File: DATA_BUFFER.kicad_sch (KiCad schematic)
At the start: 9 parts, among them IC301 ${DEVICE}

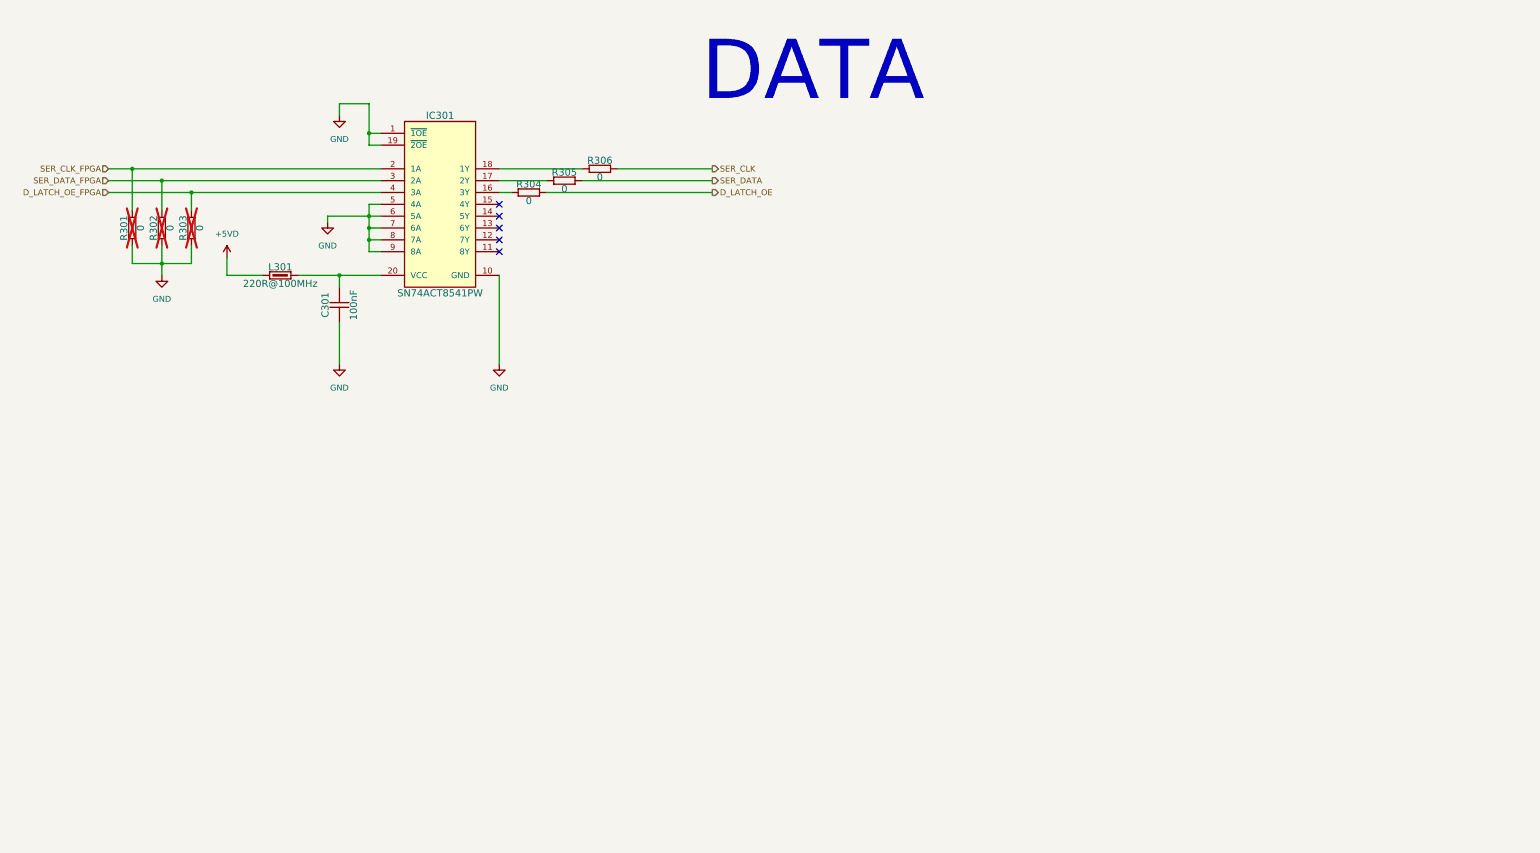
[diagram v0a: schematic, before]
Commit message: WIP snapshot
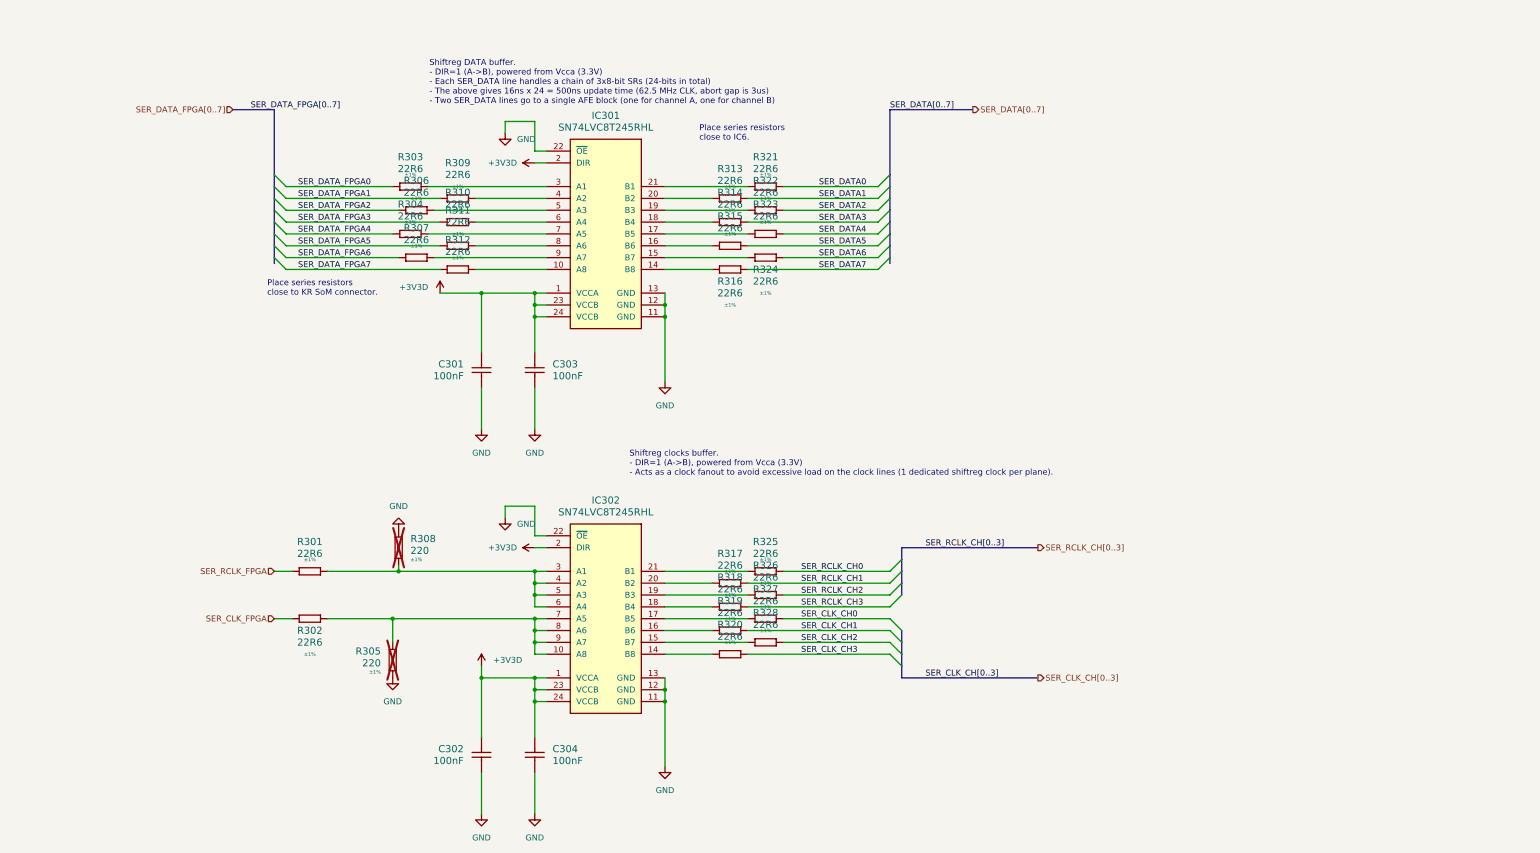
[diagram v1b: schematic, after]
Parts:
- removed IC301: ${DEVICE}, ICs And Semiconductors SMD:SOP65P640X120-20N, symbol CERN:Standard Logic/SN74ACT8541PW
- removed L301: 220R@100MHz, Inductors SMD:INDC1608X95N, symbol CERN:Inductors SMD/IND0603_MURATA_BLM18SG221TN1 [alt]
- removed R301, R302, R303, R304, R305, R306: 0, Resistors SMD:RESC1005X40N, symbol CERN:Resistors SMD/R0402_0R_JUMPER
- added C301, C302, C304: 100nF, Capacitors SMD:CAPC1005X55N, symbol CERN:Capacitors SMD/CC0402_100NF_25V_10%_X7R_YUDEN_TMK105B7104KVHF
- added IC301, IC302: ${DEVICE}, ICs And Semiconductors SMD:TEXAS_RHL (S-PVQFN-N24), symbol CERN_Linux:Standard Logic/SN74LVC8T245RHL
- added R301, R302, R303, R304, R306, R307, R309, R310, R311, R312, R313, R314, R315, R316, R317, R318, R319, R320, R321, R322, R323, R324, R325, R326, R327, R328: 22R6, Resistors SMD:RESC1005X40N, symbol CERN:Resistors SMD/R0402_22R6_1%_0.063W_100PPM
- added R305, R308: 220, Resistors SMD:RESC1005X40N, symbol CERN:Resistors SMD/R0402_220R_1%_0.0625W_100PPM
- renumbered C301 to C303
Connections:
- net GND: now also C301.1, C302.1, C304.1, IC301.11 (GND), IC301.12 (GND), IC301.13 (GND), IC301.22 (~{OE}), IC302.11 (GND), IC302.12 (GND), IC302.13 (GND), IC302.22 (~{OE}), R305.1, R308.1
- net SER_CLK_FPGA: now also R302.1
- net +3V3D: now reaches C303.2
- net +3V3D: now also C301.2, C302.2, C304.2, IC301.1 (VCCA), IC301.2 (DIR), IC301.23 (VCCB), IC301.24 (VCCB), IC302.1 (VCCA), IC302.2 (DIR), IC302.23 (VCCB), IC302.24 (VCCB)
- new net: IC302.10 (A8), IC302.7 (A5), IC302.8 (A6), IC302.9 (A7), R302.2, R305.2
- new net: IC301.9 (A7), R307.2
- new net: IC301.8 (A6), R311.2
- new net: IC301.3 (A1), R303.2
- new net: IC301.20 (B2), R313.1
- new net: IC301.21 (B1), R321.1
- new net: IC302.21 (B1), R325.1
- new net: IC301.14 (B8), R316.1
- new net: IC302.3 (A1), IC302.4 (A2), IC302.5 (A3), IC302.6 (A4), R301.2, R308.2
- new net: IC301.17 (B5), R323.1
- new net: IC302.16 (B6), R319.1
- new net: IC301.5 (A3), R306.2
- new net: IC301.18 (B4), R314.1
- new net: IC302.14 (B8), R320.1
- new net: IC302.15 (B7), R328.1
- new net: IC302.17 (B5), R327.1
- new net: IC302.18 (B4), R318.1
- new net: IC302.19 (B3), R326.1
- new net: IC302.20 (B2), R317.1
- new net: IC301.10 (A8), R312.2
- new net: IC301.6 (A4), R310.2
- new net: IC301.19 (B3), R322.1
- new net: IC301.4 (A2), R309.2
- new net: IC301.15 (B7), R324.1
- new net: IC301.16 (B6), R315.1
- new net: IC301.7 (A5), R304.2
- new net SER_CLK_CH0: R327.2
- new net SER_CLK_CH1: R319.2
- new net SER_CLK_CH2: R328.2
- new net SER_CLK_CH3: R320.2
- new net SER_DATA0: R321.2
- new net SER_DATA1: R313.2
- new net SER_DATA2: R322.2
- new net SER_DATA3: R314.2
- new net SER_DATA4: R323.2
- new net SER_DATA5: R315.2
- new net SER_DATA6: R324.2
- new net SER_DATA7: R316.2
- new net SER_DATA_FPGA0: R303.1
- new net SER_DATA_FPGA1: R309.1
- new net SER_DATA_FPGA2: R306.1
- new net SER_DATA_FPGA3: R310.1
- new net SER_DATA_FPGA4: R304.1
- new net SER_DATA_FPGA5: R311.1
- new net SER_DATA_FPGA6: R307.1
- new net SER_DATA_FPGA7: R312.1
- new net SER_RCLK_CH0: R325.2
- new net SER_RCLK_CH1: R317.2
- new net SER_RCLK_CH2: R326.2
- new net SER_RCLK_CH3: R318.2
- new net SER_RCLK_FPGA: R301.1
- no-connect marks 5 -> 0
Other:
- note added: "Place series resistors close to IC6."
- note added: "Place series resistors close to KR SoM connector."
- note added: "Shiftreg DATA buffer. - DIR=1 (A->B), powered from Vcca (3.3V) - Each SER_DATA line handles a chain of 3x8-bit SRs (24-bits in total) - The above gives 16ns x 24 = 500ns update time (62.5 MHz CLK, abort gap is 3us) - Two SER_DATA lines go to a single AFE block (one for channel A, one for channel B)"
- note added: "Shiftreg clocks buffer. - DIR=1 (A->B), powered from Vcca (3.3V) - Acts as a clock fanout to avoid excessive load on the clock lines (1 dedicated shiftreg clock per plane)."
- note removed: "DATA"
- moved on the sheet: C303

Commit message: Update project files and backups
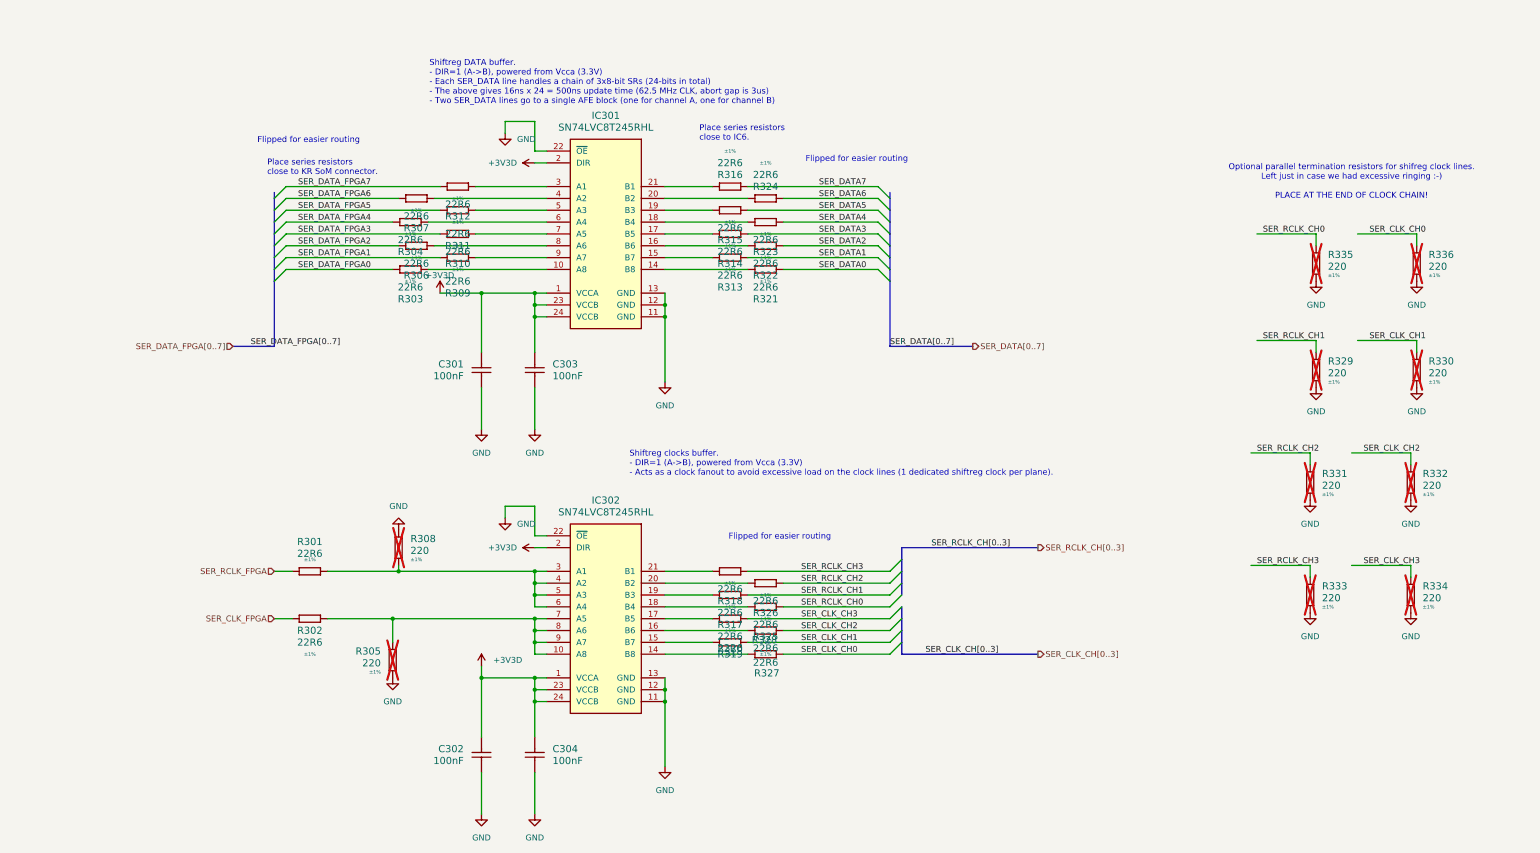
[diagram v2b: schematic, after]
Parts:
- added R329, R330, R331, R332, R333, R334, R335, R336: 220, Resistors SMD:RESC1005X40N, symbol CERN:Resistors SMD/R0402_220R_1%_0.0625W_100PPM
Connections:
- net GND: now also R329.1, R330.1, R331.1, R332.1, R333.1, R334.1, R335.1, R336.1
- net SER_CLK_CH0: now also R336.2
- net SER_CLK_CH1: now also R330.2
- net SER_CLK_CH2: now also R332.2
- net SER_CLK_CH3: now also R334.2
- net SER_RCLK_CH0: now also R335.2
- net SER_RCLK_CH1: now also R329.2
- net SER_RCLK_CH2: now also R331.2
- net SER_RCLK_CH3: now also R333.2
- net at R307.2: now also IC301.4 (A2); no longer IC301.9 (A7)
- net at R311.2: now also IC301.5 (A3); no longer IC301.8 (A6)
- net at R303.2: now also IC301.10 (A8); no longer IC301.3 (A1)
- net at R313.1: now also IC301.15 (B7); no longer IC301.20 (B2)
- net at R321.1: now also IC301.14 (B8); no longer IC301.21 (B1)
- net at R325.1: now also IC302.18 (B4); no longer IC302.21 (B1)
- net at R316.1: now also IC301.21 (B1); no longer IC301.14 (B8)
- net at R323.1: now also IC301.18 (B4); no longer IC301.17 (B5)
- net at R319.1: now also IC302.15 (B7); no longer IC302.16 (B6)
- net at R306.2: now also IC301.8 (A6); no longer IC301.5 (A3)
- net at R314.1: now also IC301.17 (B5); no longer IC301.18 (B4)
- net at IC302.14 (B8): now also R327.1; no longer R320.1
- net at R328.1: now also IC302.16 (B6); no longer IC302.15 (B7)
- net at IC302.17 (B5): now also R320.1; no longer R327.1
- net at R318.1: now also IC302.21 (B1); no longer IC302.18 (B4)
- net at IC302.19 (B3): now also R317.1; no longer R326.1
- net at IC302.20 (B2): now also R326.1; no longer R317.1
- net at R312.2: now also IC301.3 (A1); no longer IC301.10 (A8)
- net at R310.2: now also IC301.7 (A5); no longer IC301.6 (A4)
- net at R322.1: now also IC301.16 (B6); no longer IC301.19 (B3)
- net at R309.2: now also IC301.9 (A7); no longer IC301.4 (A2)
- net at R324.1: now also IC301.20 (B2); no longer IC301.15 (B7)
- net at R315.1: now also IC301.19 (B3); no longer IC301.16 (B6)
- net at R304.2: now also IC301.6 (A4); no longer IC301.7 (A5)
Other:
- note added: "Flipped for easier routing"
- note added: "Optional parallel termination resistors for shifreg clock lines. Left just in case we had excessive ringing :-) PLACE AT THE END OF CLOCK CHAIN!"
- moved on the sheet: R303, R304, R306, R307, R309, R310, R311, R312, R313, R314, R315, R316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
